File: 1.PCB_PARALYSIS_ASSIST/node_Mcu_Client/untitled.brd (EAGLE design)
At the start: 101.6 x 64.4 mm, 31 parts, among them IC2 7805TV, J1 1776118-3, J2 1776118-3, J3 1776118-3, K1 G5LE, K2 G5LE, K3 G5LE, U1 ZC563900

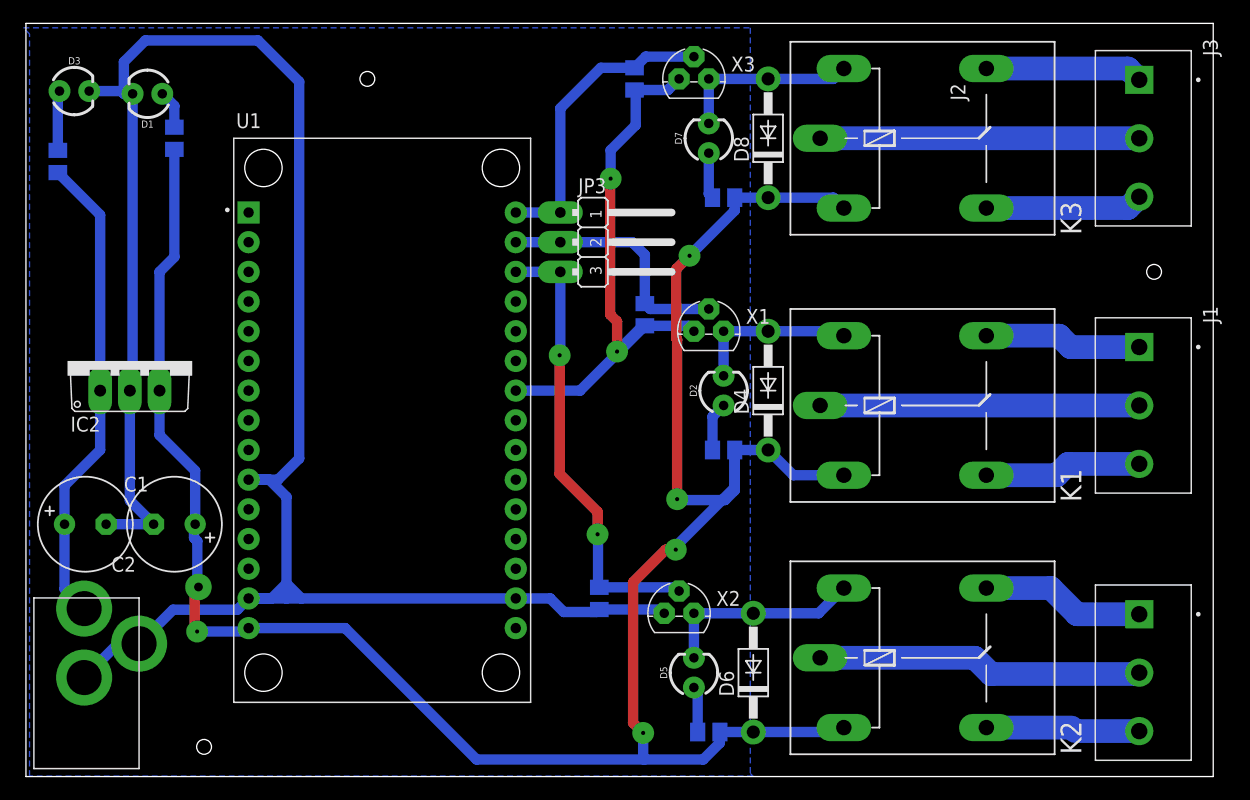
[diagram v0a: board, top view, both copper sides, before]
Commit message: updated pic of pcb
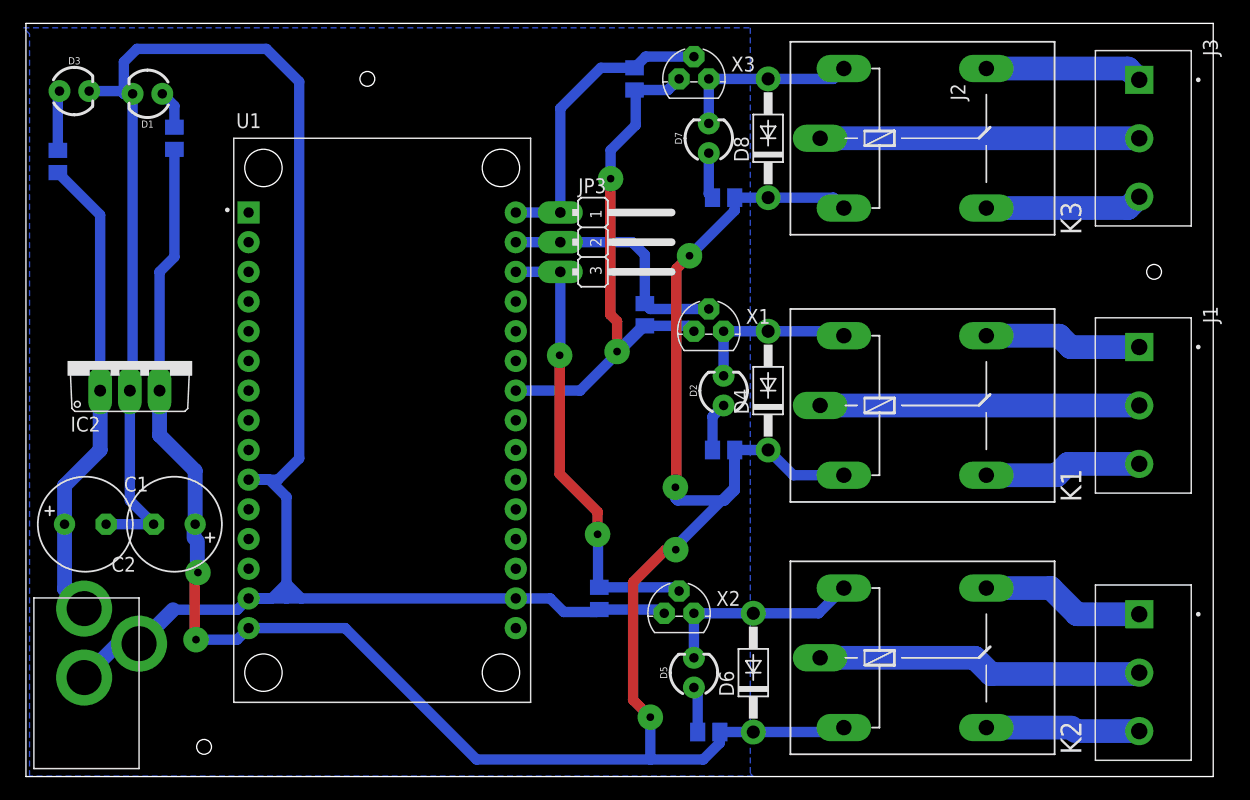
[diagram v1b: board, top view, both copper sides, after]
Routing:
- net 5V: track 192.7 -> 194.0 mm
- net GND: track 222.8 -> 222.2 mm
